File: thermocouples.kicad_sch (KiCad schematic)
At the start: 4 parts, among them U2 MAX31865xTP, U3 MAX31865xTP, U4 MAX31865xTP, U5 MAX31865xTP

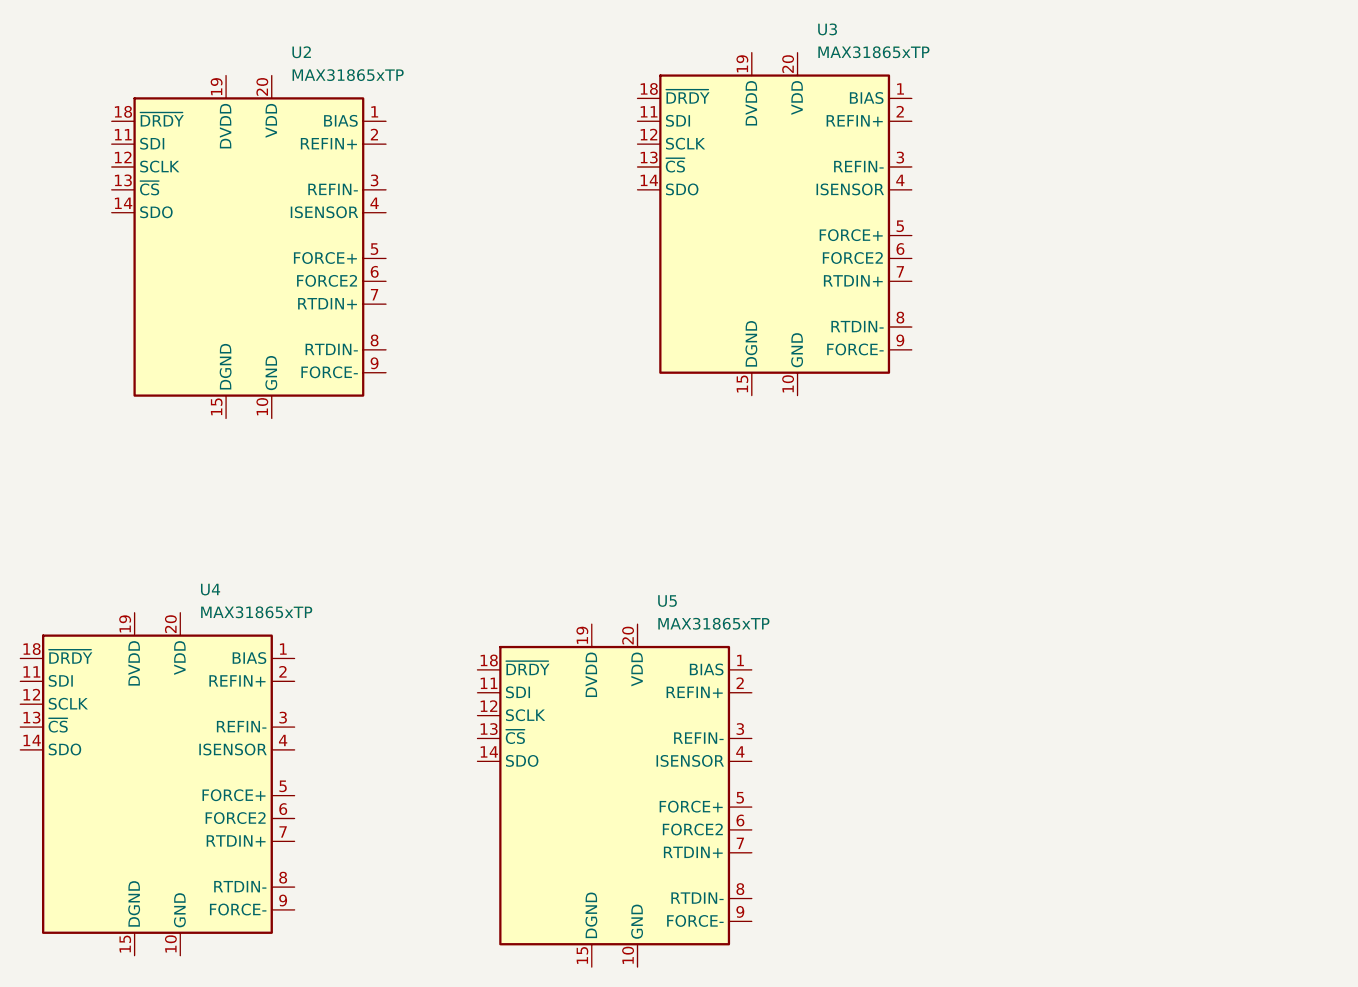
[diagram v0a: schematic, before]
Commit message: I dont know whats going on here
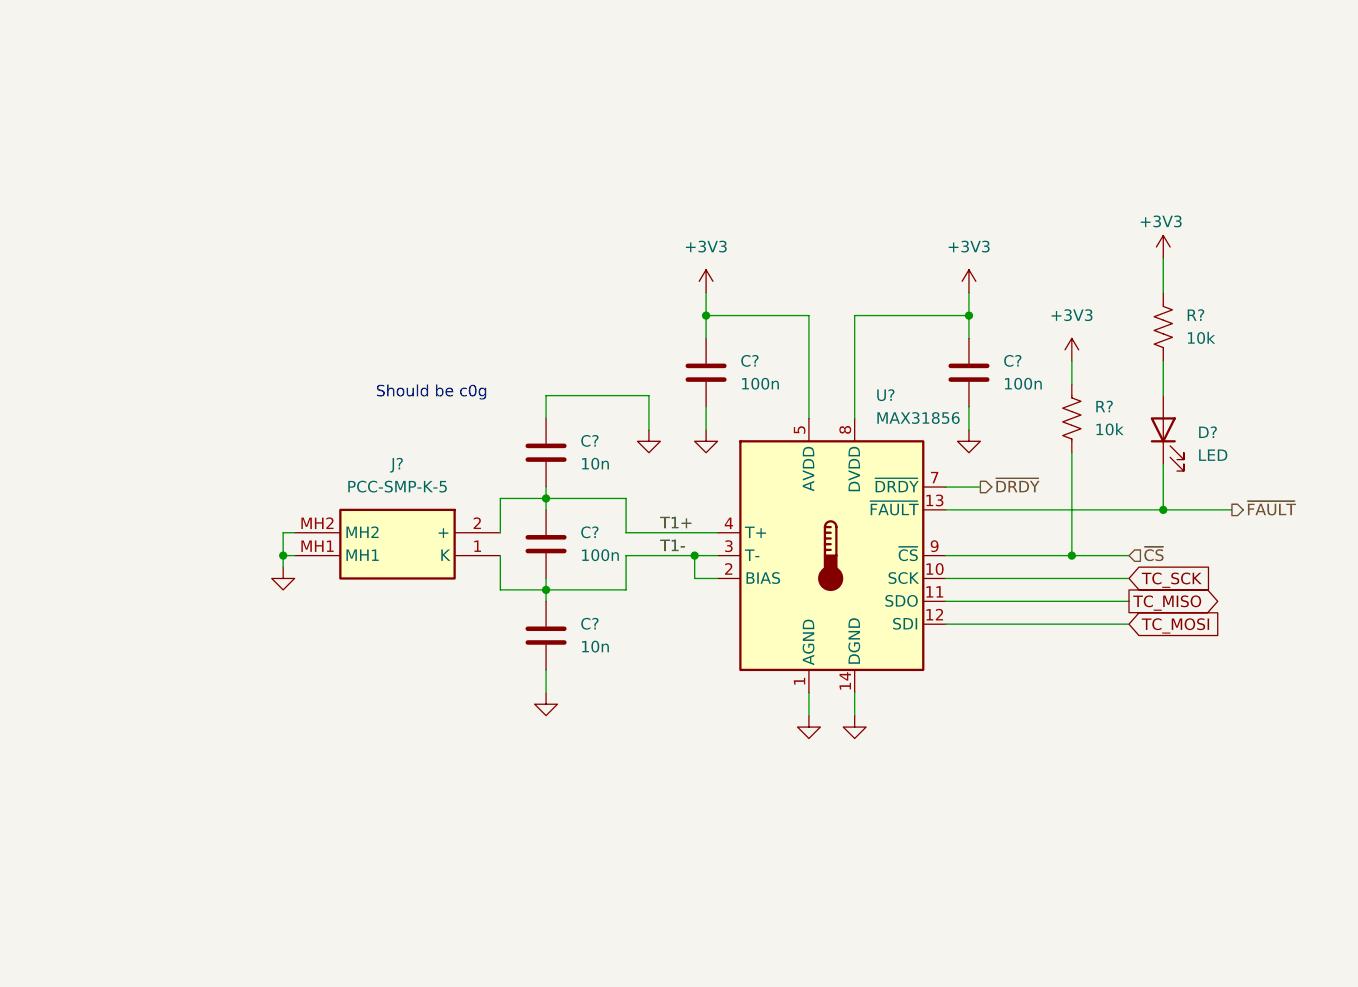
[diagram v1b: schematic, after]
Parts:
- removed U2, U3, U4, U5: MAX31865xTP, Package_DFN_QFN:TQFN-20-1EP_5x5mm_P0.65mm_EP3.25x3.25mm, symbol Sensor_Temperature:MAX31865xTP
- added C? (x3): 100n, Library:C_0402_1005Metric, symbol Device:C
- added C? (x2): 10n, Library:C_0402_1005Metric, symbol Device:C
- added D?: LED, LED_SMD:LED_0402_1005Metric, symbol Device:LED
- added J?: PCC-SMP-K-5, Omega:PCCSMPK5, symbol PCC-SMP-K-5:PCC-SMP-K-5
- added R? (x2): 10k, Library:R_0402_1005Metric, symbol Device:R_US
- added U?: MAX31856, Package_SO:TSSOP-14_4.4x5mm_P0.65mm, symbol MAX31856TriState:MAX31856
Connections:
- new net: D?.2 (A), R?.2
- new net +3V3: C?.1, C?.1, R?.1, R?.1, U?.5 (AVDD), U?.8 (DVDD)
- new net GND: C?.1, C?.2, C?.2, C?.2, J?.MH1, J?.MH2, U?.1 (AGND), U?.14 (DGND)
- new net T1+: C?.1, C?.2, J?.2 (+), U?.4 (T+)
- new net T1-: C?.1, C?.2, J?.1 (K), U?.2 (BIAS), U?.3 (T-)
- new net TC_MISO: U?.11 (SDO)
- new net TC_MOSI: U?.12 (SDI)
- new net TC_SCK: U?.10 (SCK)
- new net ~{CS}: R?.2, U?.9 (~{CS})
- new net ~{DRDY}: U?.7 (~{DRDY})
- new net ~{FAULT}: D?.1 (K), U?.13 (~{FAULT})
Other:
- note added: "Should be c0g"
